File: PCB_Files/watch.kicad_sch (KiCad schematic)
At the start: 39 parts, among them J1 USB_C_Receptacle_USB2.0_16P, Q1 BC847, Q2 BC847, SW1 SW_Push, U1 APS6404L-3SQRx-ZR, U2 ESP32-PICO-D4, U3 CP2102N-Axx-xQFN28, Y1 SG-3030CM

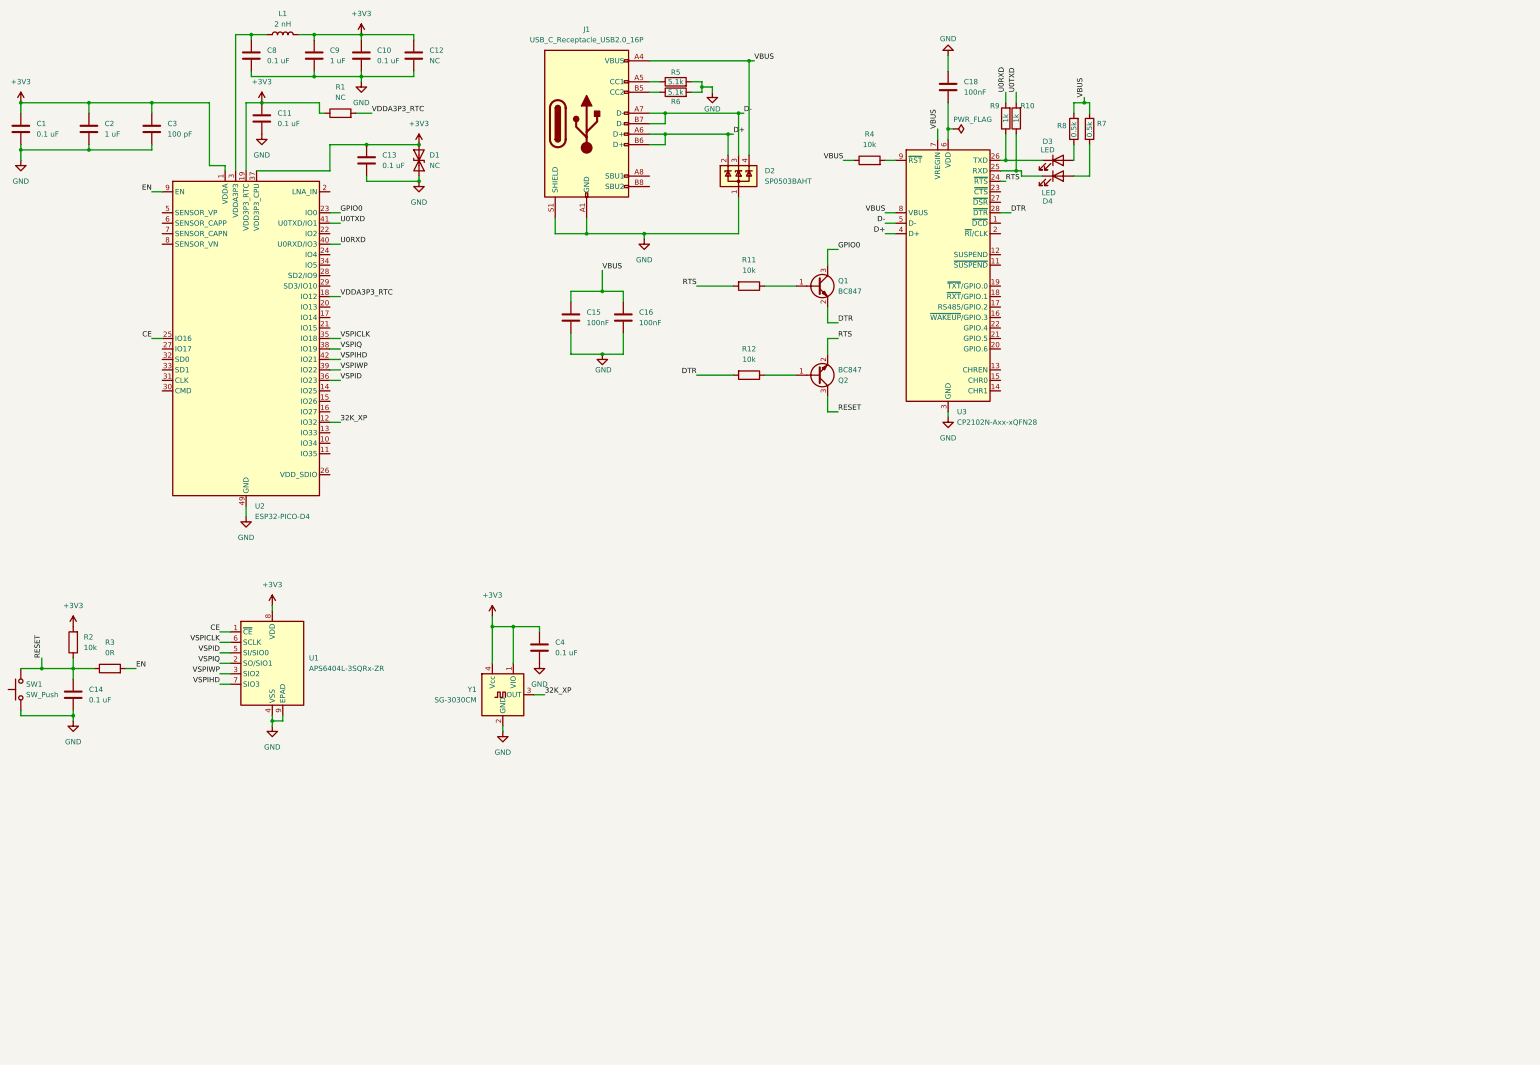
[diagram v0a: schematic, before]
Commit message: Schematics Updated
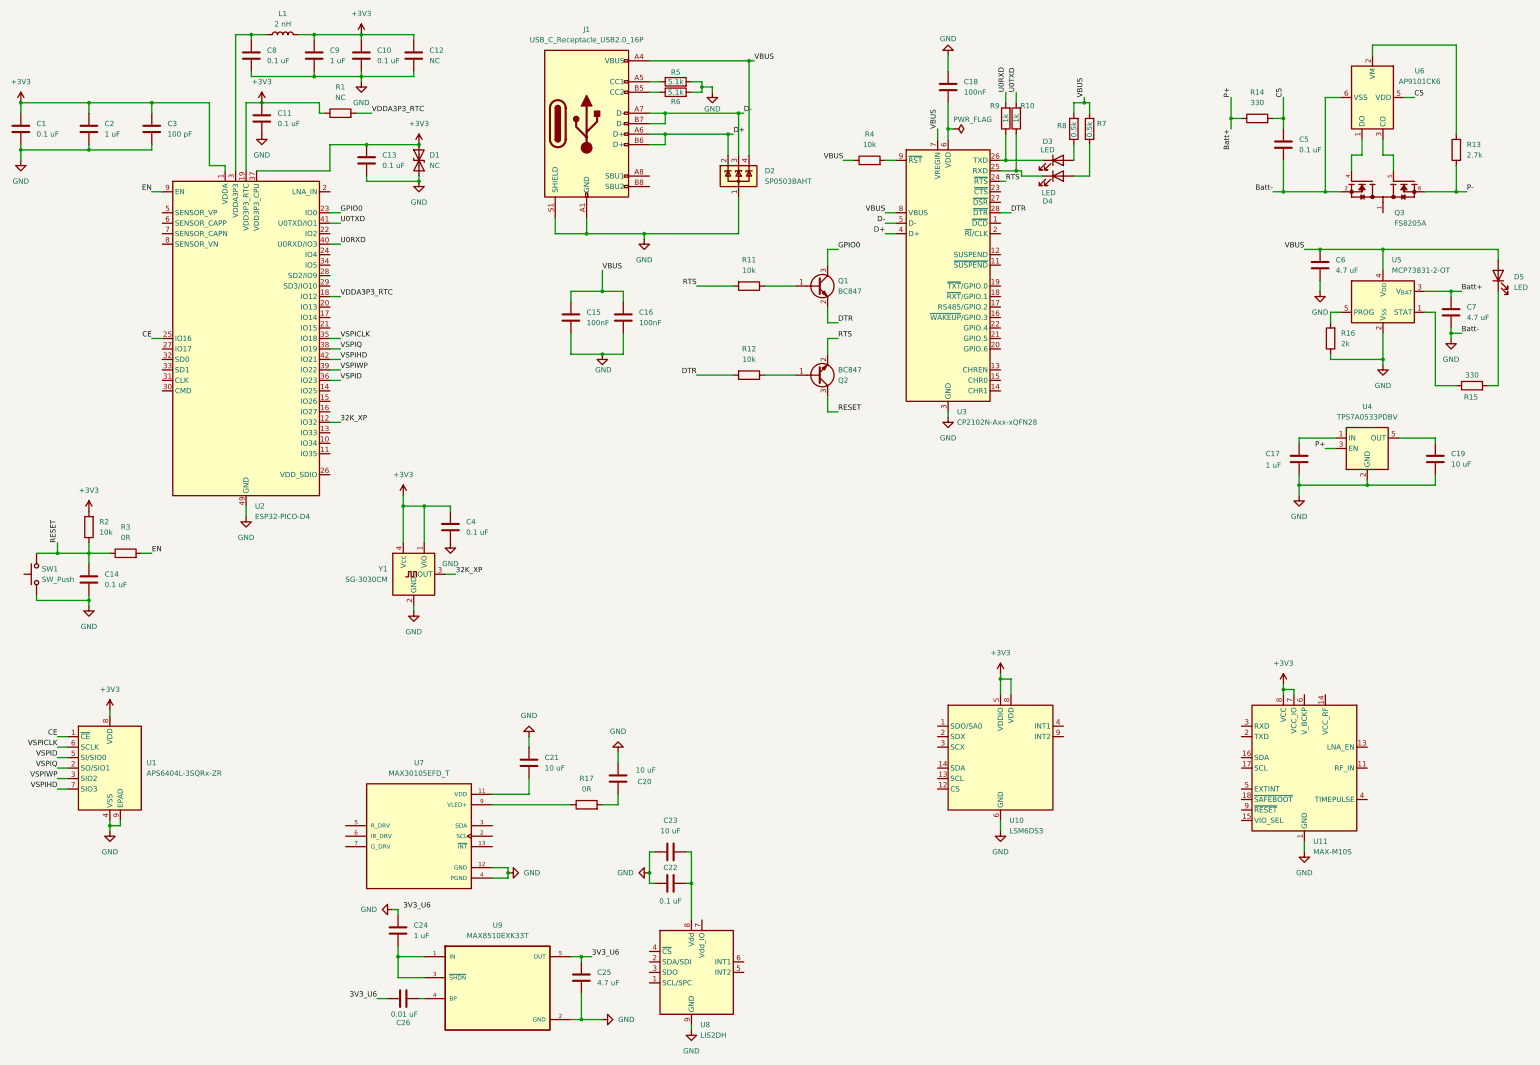
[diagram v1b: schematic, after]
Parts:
- added C17, C24: 1 uF, symbol Device:C
- added C19, C20, C21, C23: 10 uF, symbol Device:C
- added C22, C5: 0.1 uF, symbol Device:C
- added C25, C6, C7: 4.7 uF, symbol Device:C
- added C26: 0.01 uF, symbol Device:C
- added D5: LED, symbol Device:LED
- added Q3: FS8205A, symbol FS8205A:FS8205A
- added R13: 2.7k, symbol Device:R
- added R14, R15: 330, symbol Device:R
- added R16: 2k, symbol Device:R
- added R17: 0R, symbol Device:R
- added U10: LSM6DS3, Package_LGA:LGA-14_3x2.5mm_P0.5mm_LayoutBorder3x4y, symbol Sensor_Motion:LSM6DS3
- added U11: MAX-M10S, RF_GPS:ublox_MAX, symbol RF_GPS:MAX-M10S
- added U4: TPS7A0533PDBV, Package_TO_SOT_SMD:SOT-23-5, symbol Regulator_Linear:TPS7A0533PDBV
- added U5: MCP73831-2-OT, Package_TO_SOT_SMD:SOT-23-5, symbol Battery_Management:MCP73831-2-OT
- added U6: AP9101CK6, Package_TO_SOT_SMD:SOT-23-6, symbol Battery_Management:AP9101CK6
- added U7: MAX30105EFD_T, Library:14-OESIP, symbol MAX30105EFD_T:MAX30105EFD_T
- added U8: LIS2DH, Package_LGA:LGA-14_2x2mm_P0.35mm_LayoutBorder3x4y, symbol Sensor_Motion:LIS2DH
- added U9: MAX8510EXK33T, Library:SOT65P210X110-5N, symbol MAX8510EXK33T:MAX8510EXK33T
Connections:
- net +3V3: now also U10.5 (VDDIO), U10.8 (VDD), U11.7 (VCC_IO), U11.8 (VCC)
- net GND: now also C17.2, C19.2, C20.2, C21.1, C22.1, C23.1, C24.1, C25.2, C5.2, C6.2, C7.2, Q3.2, Q3.3, R16.1, U10.6 (GND), U10.7 (GND), U11.1 (GND), U11.10 (GND), U11.12 (GND), U4.2 (GND), U5.2 (V_{SS}), U6.6 (VSS), U7.12 (GND), U7.4 (PGND), U8.10 (GND), U8.11 (GND), U8.12 (GND), U8.13 (GND), U8.14 (GND), U8.9 (GND), U9.2 (GND)
- net VBUS: now also C6.1, D5.2 (A), U5.4 (V_{DD})
- new net: R15.1, U5.1 (STAT)
- new net: D5.1 (K), R15.2
- new net: C17.1, U4.1 (IN)
- new net: C22.2, C23.2, U8.8 (Vdd)
- new net: C20.1, R17.2
- new net: R16.2, U5.5 (PROG)
- new net: R17.1, U7.9 (VLED+)
- new net: C24.2, U9.1 (IN), U9.3 (~{SHDN})
- new net: C26.2, U9.4 (BP)
- new net: C19.1, U4.5 (OUT)
- new net: C21.2, U7.11 (VDD)
- new net: R13.2, U6.2 (VM)
- new net: Q3.4, U6.1 (DO)
- new net: Q3.5, U6.3 (CO)
- new net: Q3.1, Q3.8
- new net 3V3_U6: C25.1, C26.1, U9.5 (OUT)
- new net Batt+: C7.1, R14.1, U4.3 (EN), U5.3 (V_{BAT})
- new net C5: C5.1, R14.2, U6.5 (VDD)
- new net P-: Q3.6, Q3.7, R13.1
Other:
- moved on the sheet: C14, C4, R2, R3, SW1, U1, Y1

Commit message: Connected few peripherals and formatting
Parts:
- removed C24: 1 uF, symbol Device:C
- removed C25: 4.7 uF, symbol Device:C
- removed C26: 0.01 uF, symbol Device:C
- removed U9: MAX8510EXK33T, Library:SOT65P210X110-5N, symbol MAX8510EXK33T:MAX8510EXK33T
- added C27, C28, C29: 0.1 uF, symbol Device:C
- added C30, C31: 1uF, symbol Device:C
- added Q4, Q5: BSS138, Package_TO_SOT_SMD:SOT-23, symbol Transistor_FET:BSS138
- added R18, R19, R20, R21: 4.7k, symbol Device:R
- added U12: MCP1700x-120xxMB, Package_TO_SOT_SMD:SOT-89-3, symbol Regulator_Linear:MCP1700x-120xxMB
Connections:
- net +3V3: now also R17.1, U7.9 (VLED+), C27.1, C28.2
- net GND: now also U10.2 (SDX), U10.3 (SCX), C27.2, C28.1, C29.1, C30.1, C31.1, U12.1 (GND)
- net MISO: now reaches U10.1 (SDO/SA0)
- net MISO: now also U2.28 (SD2/IO9), U8.3 (SDO)
- net CS: now reaches U10.12 (CS)
- net CS: now also U2.21 (IO15), U8.4 (~{CS})
- net SCL: now reaches U10.13 (SCL)
- net SCL: now also U2.34 (IO5), U8.1 (SCL/SPC)
- net MOSI: now reaches U10.14 (SDA)
- net MOSI: now also U2.29 (SD3/IO10), U8.2 (SDA/SDI)
- net INTR1_IMU: now reaches U10.4 (INT1)
- net INTR1_IMU: now also U2.24 (IO4)
- net INTR2_IMU: now reaches U10.9 (INT2)
- net INTR2_IMU: now also U2.22 (IO2)
- net SDA: now reaches U2.14 (IO25)
- net SDA: now also R21.2
- net SCL_i2c: now reaches U2.27 (IO17)
- net SCL_i2c: now also R18.2
- net at U8.7 (Vdd_IO): now also C22.2, C23.2, U8.8 (Vdd)
- net 3V3: now reaches C19.1, U4.5 (OUT)
- net 3V3: now also C30.2, U12.2 (VI)
- net at C21.2, U7.11 (VDD): now also C29.2
- net LV_SCL: now reaches U7.2 (SCL)
- net LV_SCL: now also Q4.2 (S), R20.1
- net LV_SDA: now reaches U7.3 (SDA)
- net LV_SDA: now also Q5.2 (S), R19.1
- new net: Q5.3 (D), R21.1
- new net: Q4.3 (D), R18.1
- new net 1.8V: C31.2, Q4.1 (G), Q5.1 (G), R19.2, R20.2, U12.3 (VO)
- no-connect marks 0 -> 3
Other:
- note added: "Accelerometer"
- note added: "Battery Management"
- note added: "Battery Protection Module"
- note added: "Charging Module"
- note added: "Converts 3.3V to 1.8V"
- note added: "Converts 3.7V to 3.3V"
- note added: "Crystal Oscillator"
- note added: "GNSS Receiver (Incomplete)"
- note added: "IMU"
- note added: "MCU"
- note added: "Optical Sensor (Incomplete)"
- note added: "Peripherals"
- note added: "SPI/QPI PSRAM"
- note added: "Serial Boot&Switch"
- note added: "Smart Watch"
- note added: "Type-C Port"
- note added: "USB to TTL(Serial)Convertor"
- note added: "Voltage Regulator"
- moved on the sheet: C1, C10, C11, C12, C13, C14, C15, C16, C17, C18, C19, C2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

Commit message: Added Sensors
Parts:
- added C24, C25: 1 uF, symbol Device:C
- added U13: DRV2605LDGS, Package_SO:VSSOP-10_3x3mm_P0.5mm, symbol Driver_Haptic:DRV2605LDGS
- added U9: BMP388, symbol BMP388:BMP388
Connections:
- net +3V3: now also C24.1, U13.10 (VDD), U13.5 (EN), U13.6 (VDD/NC), U9.1 (VDDIO), U9.10 (VDD)
- net 1.8V: now also R20.1; no longer R20.2
- net GND: now also C24.2, C25.2, U13.4 (IN/TRIG), U13.8 (GND), U9.3 (VSS), U9.8 (VSS), U9.9 (VSS)
- net LV_SCL: now also R20.2, U13.2 (SCL); no longer R20.1
- net LV_SDA: now also U13.3 (SDA)
- new net: C25.1, U13.1 (REG)
- new net Motor_OUT+: U13.7 (OUT+)
- new net Motor_OUT-: U13.9 (OUT-)
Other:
- note added: "Barometer (incomplete)"
- note added: "DRV2605L"
- note added: "I2C Lines"
- moved on the sheet: C20, C21, C22, C23, C27, C28, C29, Q4, Q5, R17, R18, R19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
